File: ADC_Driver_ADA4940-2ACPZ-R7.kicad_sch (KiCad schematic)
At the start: 29 parts

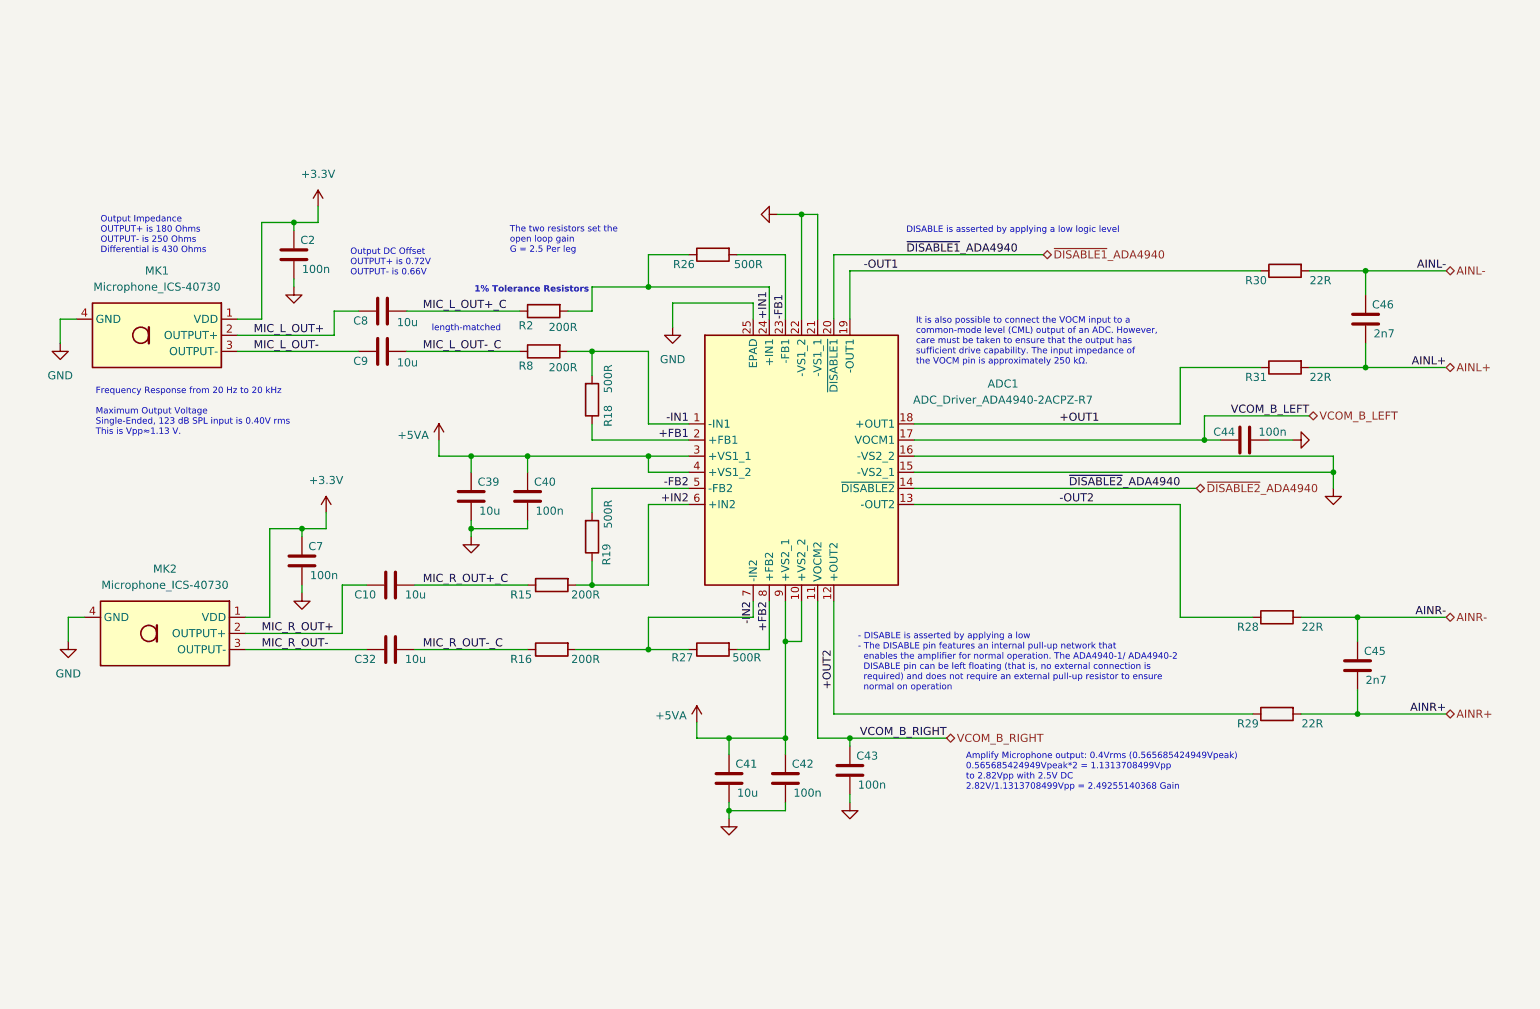
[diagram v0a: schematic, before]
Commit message: Update
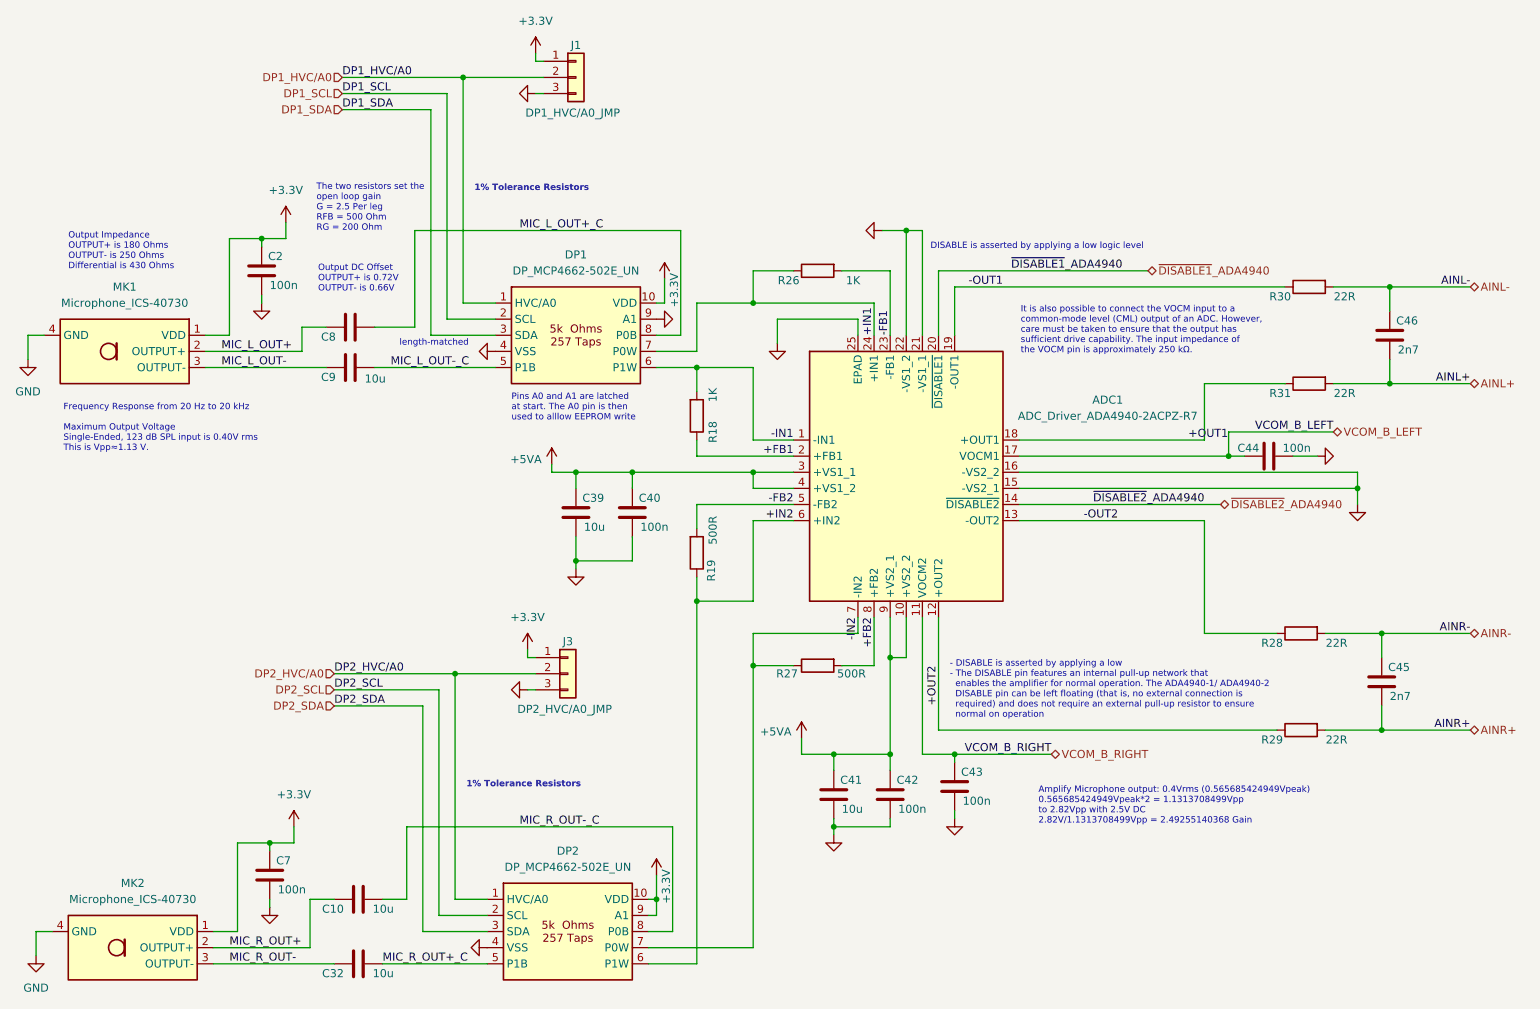
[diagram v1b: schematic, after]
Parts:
- removed R15, R16, R2, R8: 200R, Resistor_SMD:R_0805_2012Metric, symbol Device:R
- added DP1, DP2: DP_MCP4662-502E_UN, Personal_Project:DP_MCP4662_SOP50P490X110-10N, symbol Personal_Projects:DP_MCP4662-502E_UN
- added J1: DP1_HVC/A0_JMP, Connector_PinHeader_2.54mm:PinHeader_1x03_P2.54mm_Vertical, symbol Connector_Generic:Conn_01x03
- added J3: DP2_HVC/A0_JMP, Connector_PinHeader_2.54mm:PinHeader_1x03_P2.54mm_Vertical, symbol Connector_Generic:Conn_01x03
- R18, R26: value 500R -> 1K
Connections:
- net +3.3V: now also DP1.10 (VDD), DP2.10 (VDD), DP2.9 (A1), J1.1 (Pin_1), J3.1 (Pin_1)
- net +IN1: now also DP1.7 (P0W)
- net +IN2: now also DP2.6 (P1W)
- net -IN1: now also DP1.6 (P1W)
- net -IN2: now also DP2.7 (P0W)
- net GND: now also DP1.4 (VSS), DP1.9 (A1), DP2.4 (VSS), J1.3 (Pin_3), J3.3 (Pin_3)
- net MIC_L_OUT+_C: now also DP1.8 (P0B)
- net MIC_L_OUT-_C: now also DP1.5 (P1B)
- net MIC_R_OUT+_C: now also C32.2, DP2.5 (P1B); no longer C10.2
- net MIC_R_OUT-_C: now also C10.2, DP2.8 (P0B); no longer C32.2
- new net DP1_HVC/A0: DP1.1 (HVC/A0), J1.2 (Pin_2)
- new net DP1_SCL: DP1.2 (SCL)
- new net DP1_SDA: DP1.3 (SDA)
- new net DP2_HVC/A0: DP2.1 (HVC/A0), J3.2 (Pin_2)
- new net DP2_SCL: DP2.2 (SCL)
- new net DP2_SDA: DP2.3 (SDA)
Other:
- note added: "Pins A0 and A1 are latched at start. The A0 pin is then used to alllow EEPROM write"
- note added: "The two resistors set the open loop gain G = 2.5 Per leg RFB = 500 Ohm RG = 200 Ohm"
- note removed: "The two resistors set the open loop gain G = 2.5 Per leg"
- moved on the sheet: ADC1, C10, C2, C32, C39, C40, C41, C42, C43, C44, C45, C46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
